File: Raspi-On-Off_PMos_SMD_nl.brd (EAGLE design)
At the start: 52 x 28 mm, 32 parts, among them IC1 74AUC1G17, T1 FDC6327C, T2 FDC6327C, T3 BSS123, T4 IRF7416, T5 IRLML0030, X1 MKDSN1,5/2-5,08

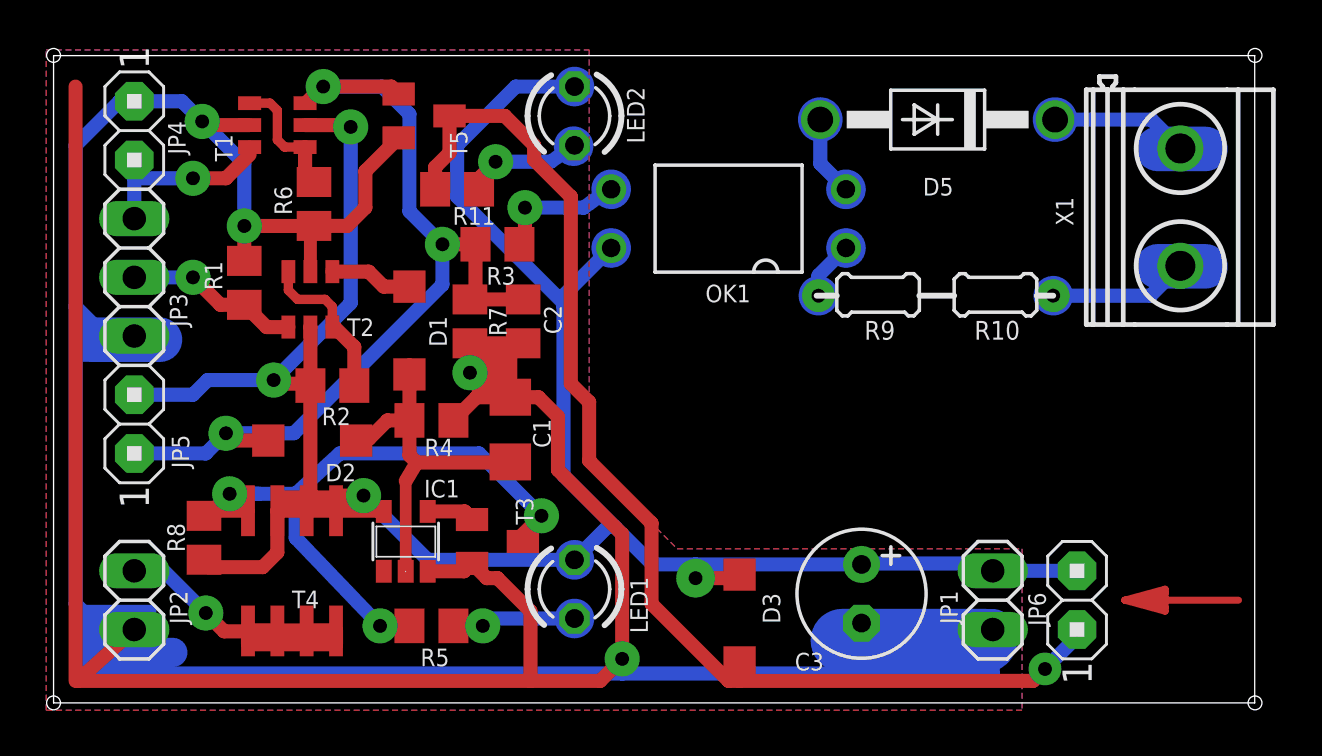
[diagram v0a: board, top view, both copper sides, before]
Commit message: Add files via upload
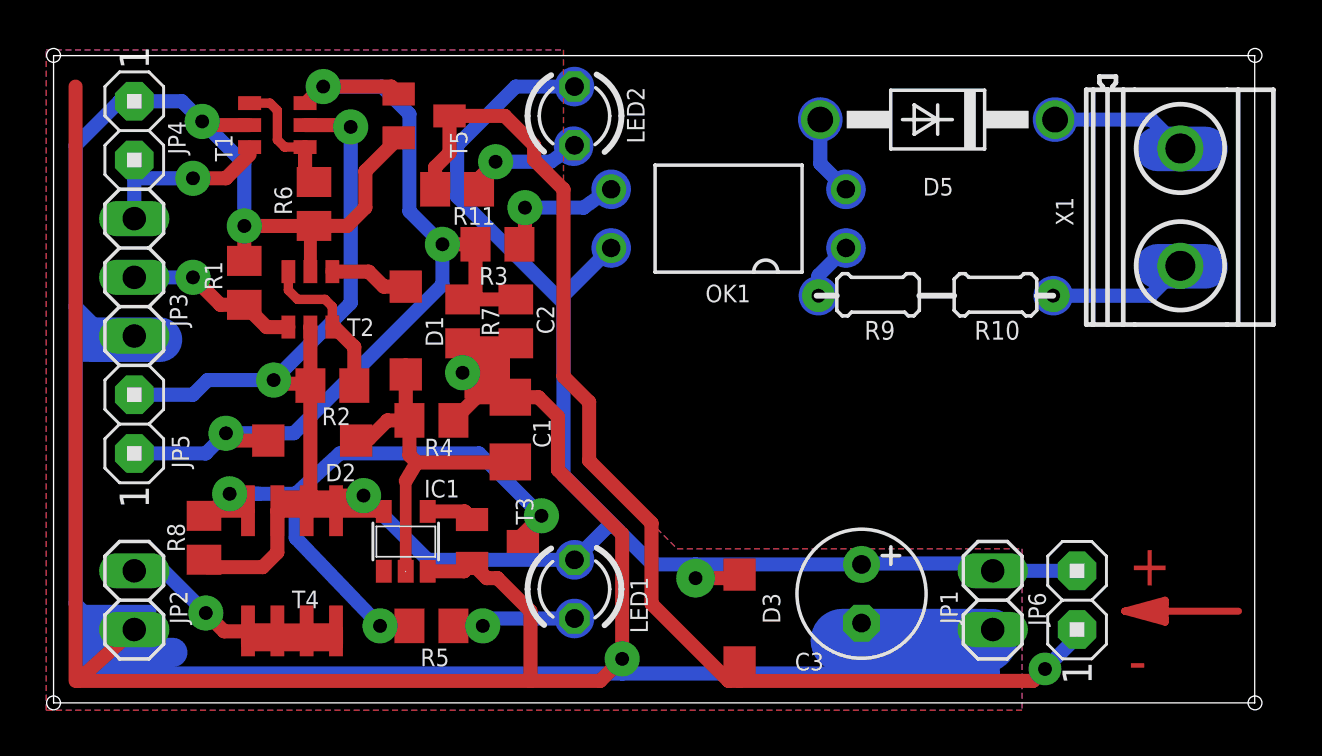
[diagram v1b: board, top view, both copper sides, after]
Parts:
- T3: value BSS123 -> IRLML2803
- moved R7 0.32 mm to (17.7, 16.5)
- moved C2 0.32 mm to (20.0, 16.5)
- moved D1 0.16 mm to (15.2, 16.1)
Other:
- board text added: "+"
- board text added: "-"
